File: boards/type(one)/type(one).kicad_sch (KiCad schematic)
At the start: 39 parts, among them J1 IDC-Header_02x03, J2 IDC-Header_02x05, J3 Conn_01x02, J4 Conn_01x05, J5 Conn_01x05, J6 Conn_01x03, J7 Conn_01x02, J8 Conn_01x02, Q1 2N2907, Q2 2n2222, Q3 IRF4905, Q4 2N7000, U1 ESP32-WROOM-UE, U2 LM393, U3 LF33_TO220, U4 LM1117T-5.0

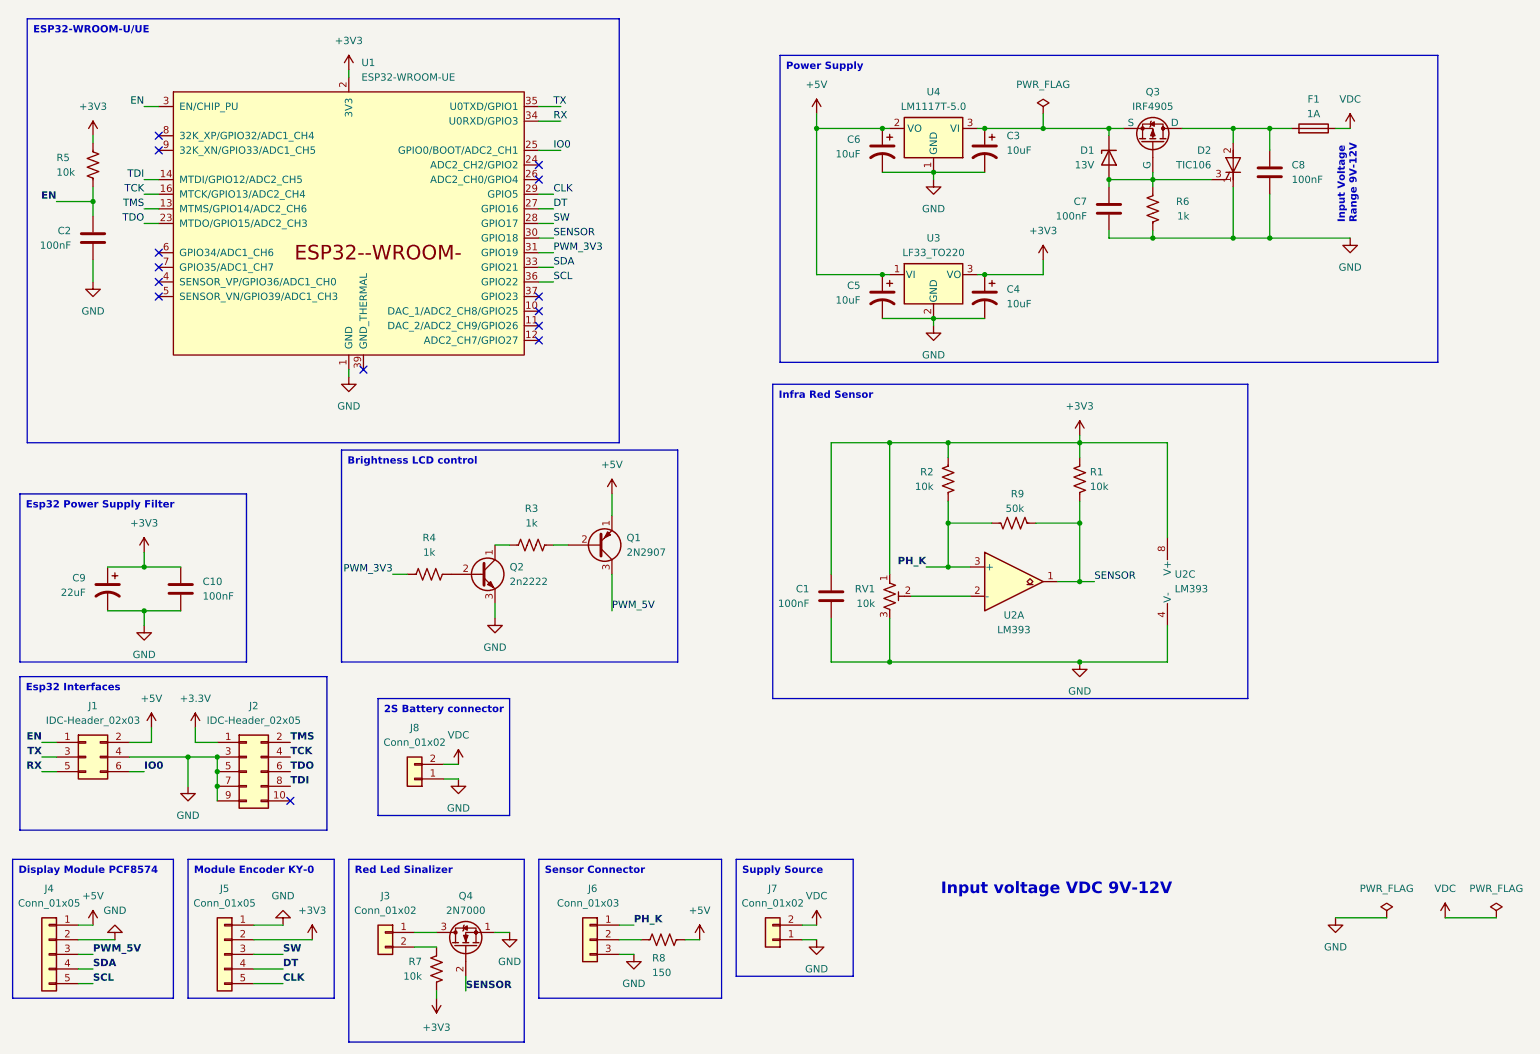
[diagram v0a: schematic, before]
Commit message: organize schematic
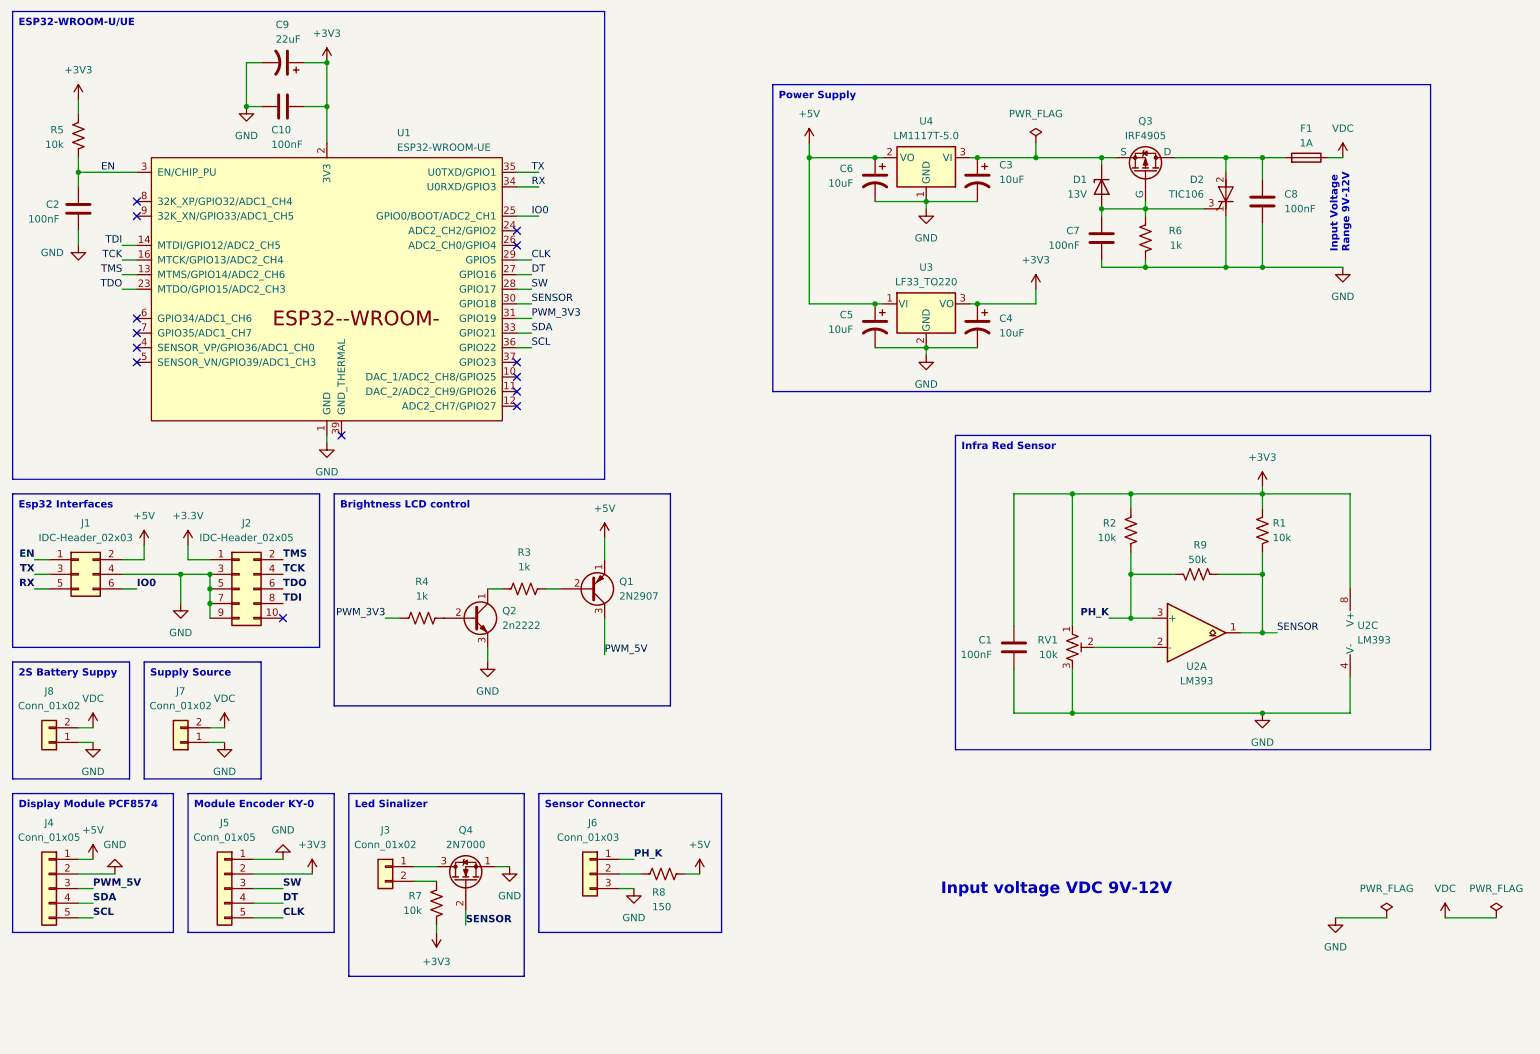
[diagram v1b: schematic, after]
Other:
- moved on the sheet: C1, C10, C2, C3, C4, C5, C6, C7, C8, C9, D1, D2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
